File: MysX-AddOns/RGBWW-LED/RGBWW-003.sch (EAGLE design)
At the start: 13 parts

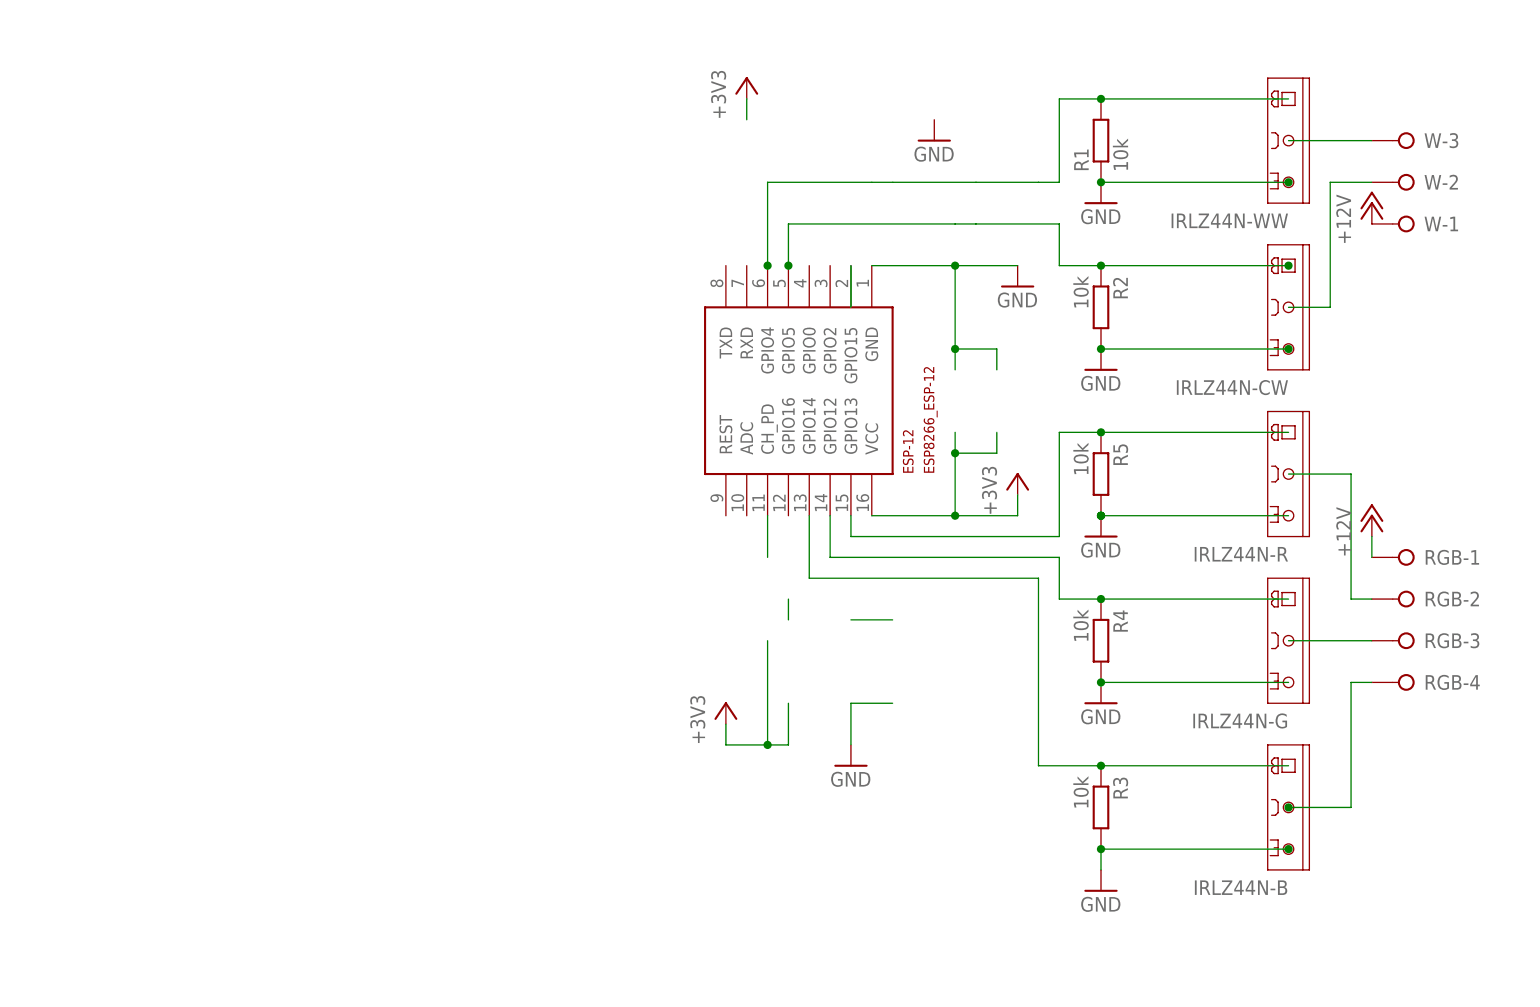
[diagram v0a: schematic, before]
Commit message: AddOns
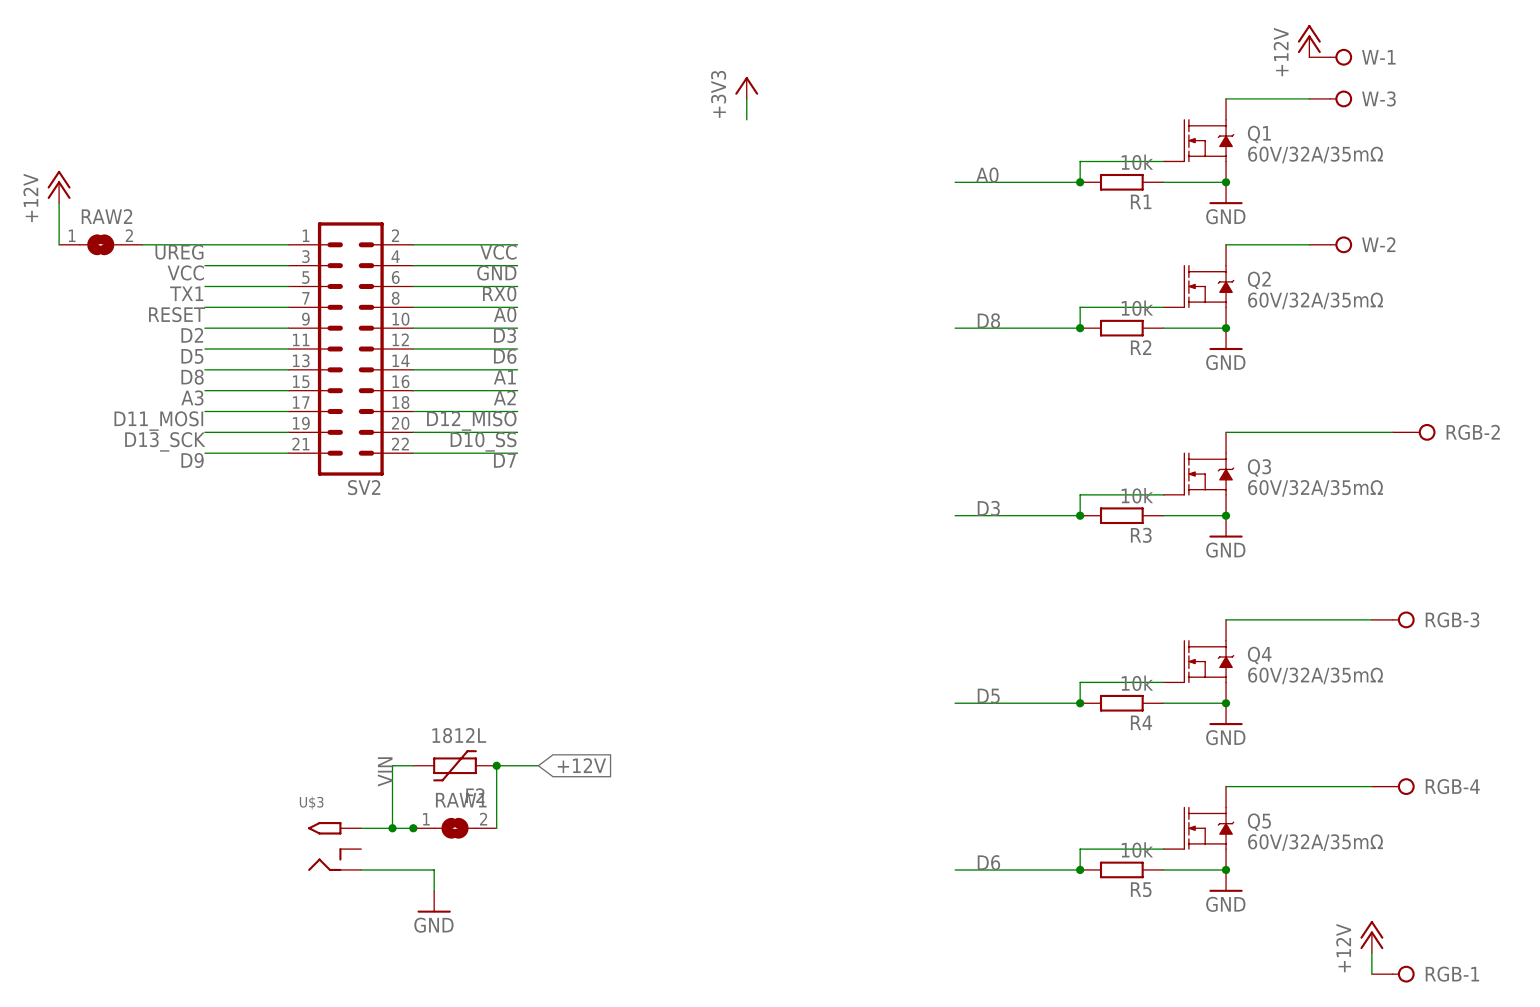
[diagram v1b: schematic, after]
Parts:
- removed ESP-12: ESP8266_ESP-12, ESP8266-ESP12:ESP8266_ESP-12
- removed IRLZ44N-B, IRLZ44N-CW, IRLZ44N-G, IRLZ44N-R, IRLZ44N-WW: TIP121, PAsystem:TIP121
- added F2: 1812L, ptc-littlefuse:1812L
- added Q1, Q2, Q3, Q4, Q5: 60V/32A/35mΩ, SparkFun-DiscreteSemi:MOSFET-NCH-FQP30N06L
- added RAW1, RAW2: (no value), jumper:SJ
- added SV2: (no value), con-Pinheader:MA11-2
- added U$3: 2.1MMJACKTHM, adafruit:2.1MMJACKTHM
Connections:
- removed net +3V3: ESP-12.VCC
- removed net N$2: ESP-12.CH_PD
- removed net N$7: ESP-12.GPIO15
- removed net RGB-B: ESP-12.GPIO14, IRLZ44N-B.B, R3.1
- removed net RGB-B-OUT: IRLZ44N-B.C, RGB-4.KL
- removed net RGB-CW: ESP-12.GPIO5, IRLZ44N-CW.B, R2.1
- removed net RGB-CW-OUT: IRLZ44N-CW.C, W-2.KL
- removed net RGB-G: ESP-12.GPIO12, IRLZ44N-G.B, R4.1
- removed net RGB-G-OUT: IRLZ44N-G.C, RGB-3.KL
- removed net RGB-R: ESP-12.GPIO13, IRLZ44N-R.B, R5.1
- removed net RGB-R-OUT: IRLZ44N-R.C, RGB-2.KL
- removed net RGB-WW: ESP-12.GPIO4, IRLZ44N-WW.B, R1.2
- new net A0: Q1.G, R1.2, SV2.8
- new net A1: SV2.14
- new net A2: SV2.16
- new net A3: SV2.15
- new net D10_SS: SV2.20
- new net D11_MOSI: SV2.17
- new net D12_MISO: SV2.18
- new net D13_SCK: SV2.19
- new net D2: SV2.9
- new net D3: Q3.G, R3.2, SV2.10
- new net D5: Q4.G, R4.2, SV2.11
- new net D6: Q5.G, R5.2, SV2.12
- new net D7: SV2.22
- new net D8: Q2.G, R2.2, SV2.13
- new net D9: SV2.21
- new net RESET: SV2.7
- new net RGB-WW-OUT1: Q2.D, W-2.KL
- new net RGB-WW-OUT2: Q3.D, RGB-2.KL
- new net RGB-WW-OUT3: Q4.D, RGB-3.KL
- new net RGB-WW-OUT4: Q5.D, RGB-4.KL
- new net RX0: SV2.6
- new net TX1: SV2.5
- new net UREG: RAW2.2, SV2.1
- new net VCC: SV2.2, SV2.3
- new net VIN: F2.2, RAW1.1, U$3.TIP
- net +12V: now also F2.1, RAW1.2, RAW2.1
- net GND: now also Q1.S, Q2.S, Q3.S, Q4.S, Q5.S, R2.1, R3.1, R4.1, R5.1, SV2.4, U$3.RING; no longer ESP-12.GND, IRLZ44N-B.E, IRLZ44N-CW.E, IRLZ44N-G.E, IRLZ44N-R.E, IRLZ44N-WW.E, R2.2, R3.2, R4.2, R5.2
- net RGB-WW-OUT: now also Q1.D; no longer IRLZ44N-WW.C
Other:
- moved on the sheet: R1, R2, R3, R4, R5, RGB-1, RGB-2, RGB-3, RGB-4, W-1, W-2, W-3
